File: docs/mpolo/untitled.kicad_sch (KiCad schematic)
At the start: 2 parts, among them J1 Raspberry_Pi_4, U1 STM32G474RETx

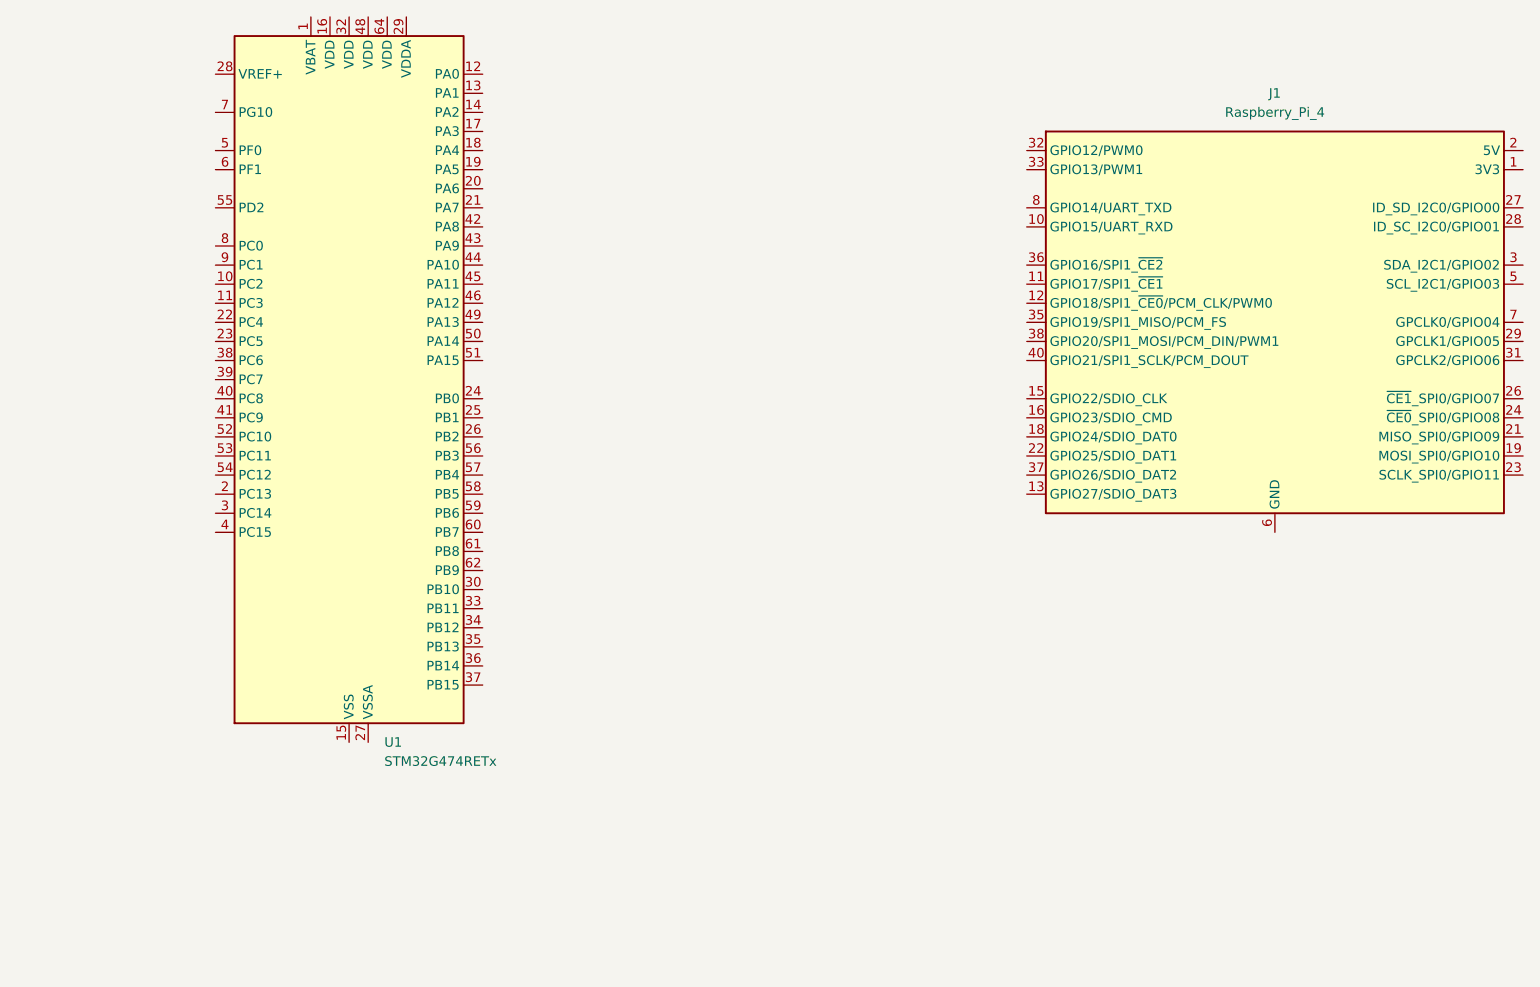
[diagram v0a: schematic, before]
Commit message: More docs and research
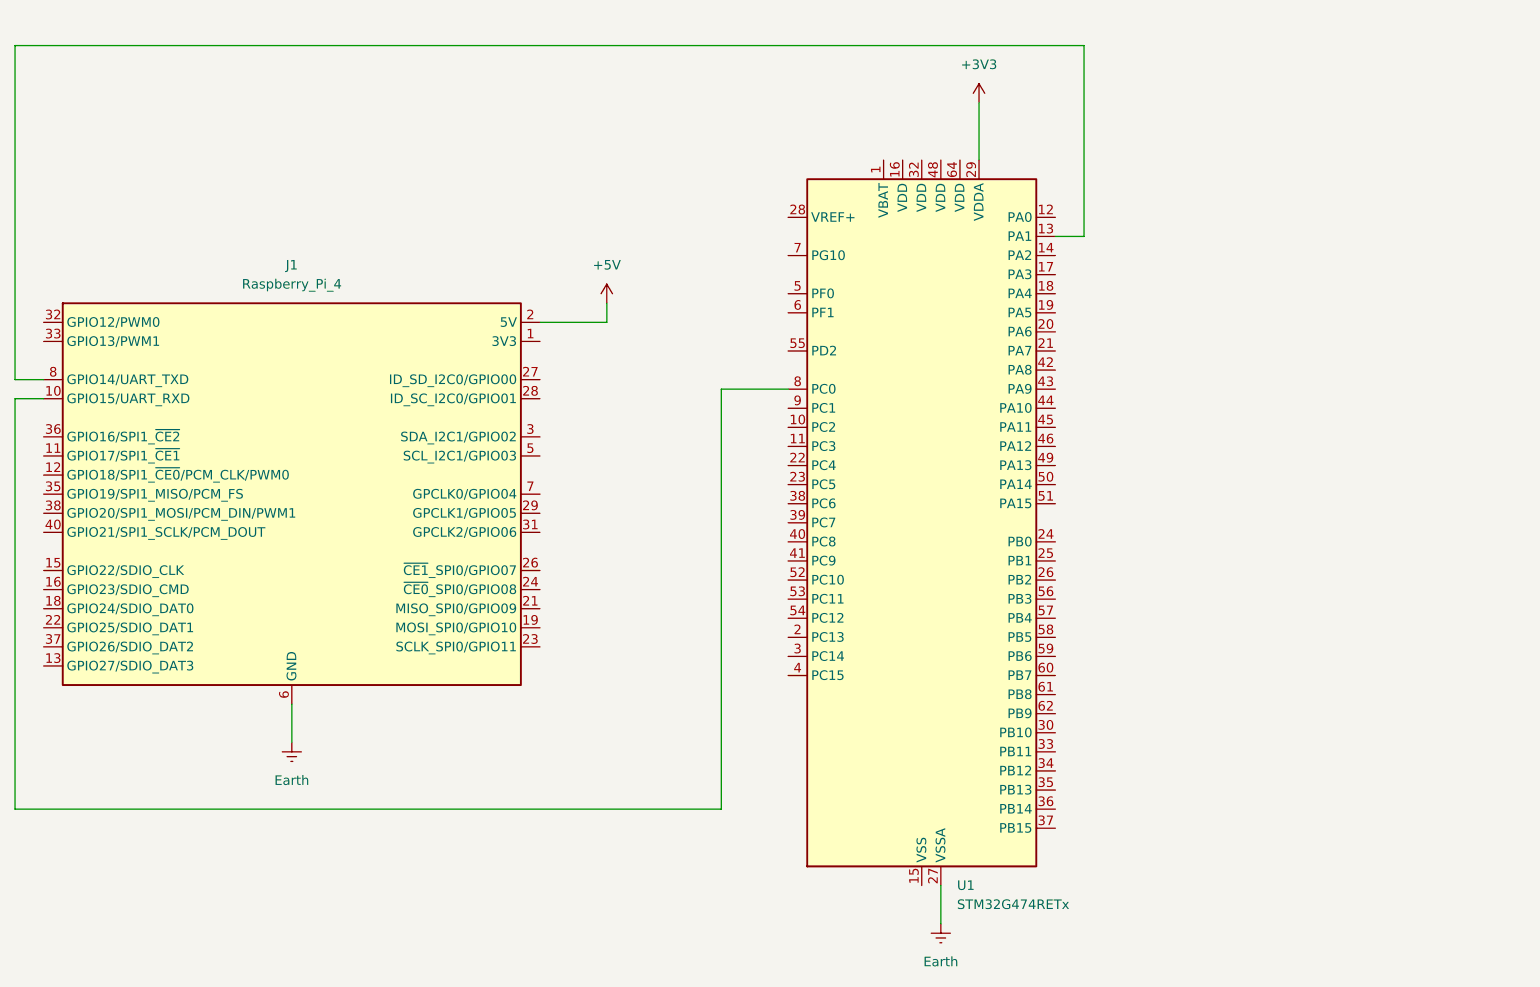
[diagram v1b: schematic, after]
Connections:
- net at J1.10 (GPIO15/UART_RXD): now also U1.8 (PC0)
- net Earth: now reaches J1.14 (GND), J1.20 (GND), J1.25 (GND), J1.30 (GND), J1.34 (GND), J1.39 (GND), J1.6 (GND), J1.9 (GND)
- net Earth: now also U1.27 (VSSA)
- net +5V: now reaches J1.2 (5V), J1.4 (5V)
- net at J1.8 (GPIO14/UART_TXD): now also U1.13 (PA1)
- net +3V3: now reaches U1.29 (VDDA)
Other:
- moved on the sheet: J1, U1
